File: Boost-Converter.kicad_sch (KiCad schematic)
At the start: 6 parts

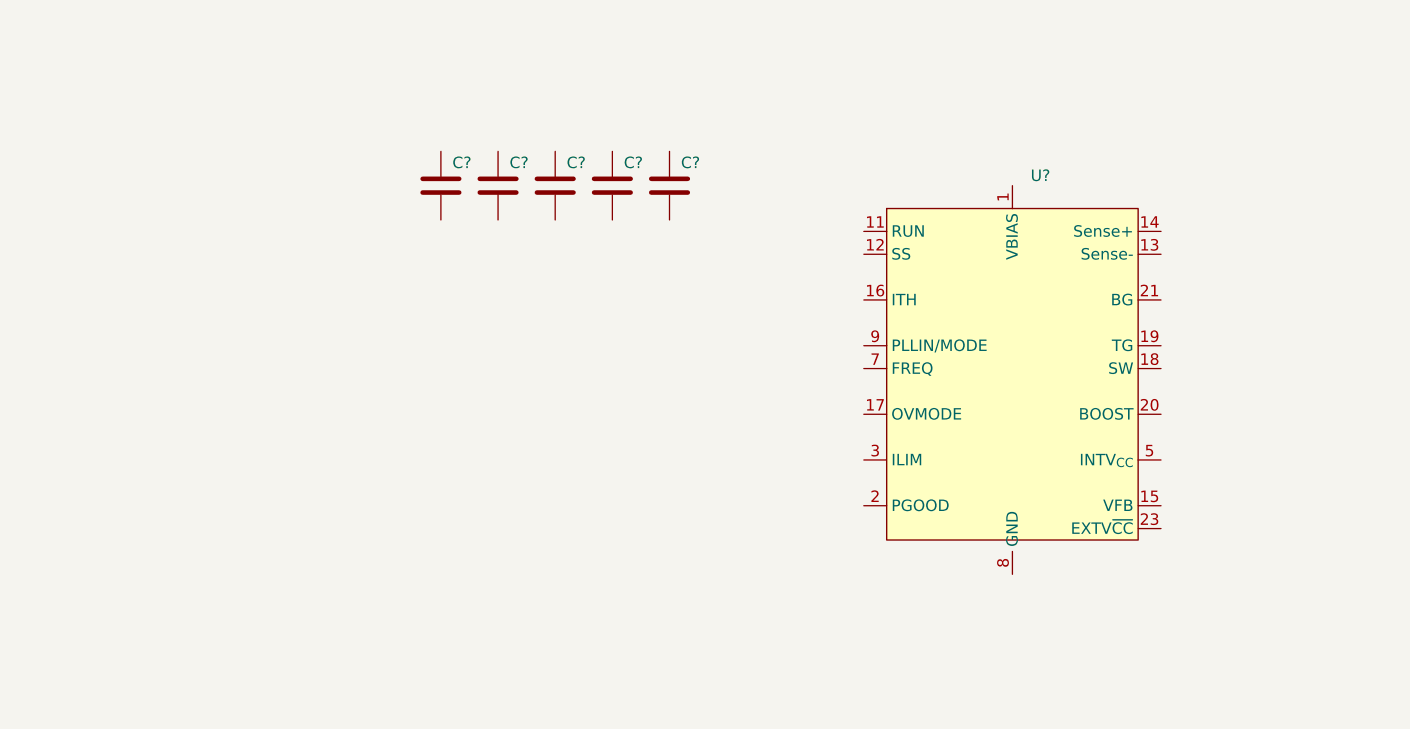
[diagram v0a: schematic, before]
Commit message: WIP boost converter
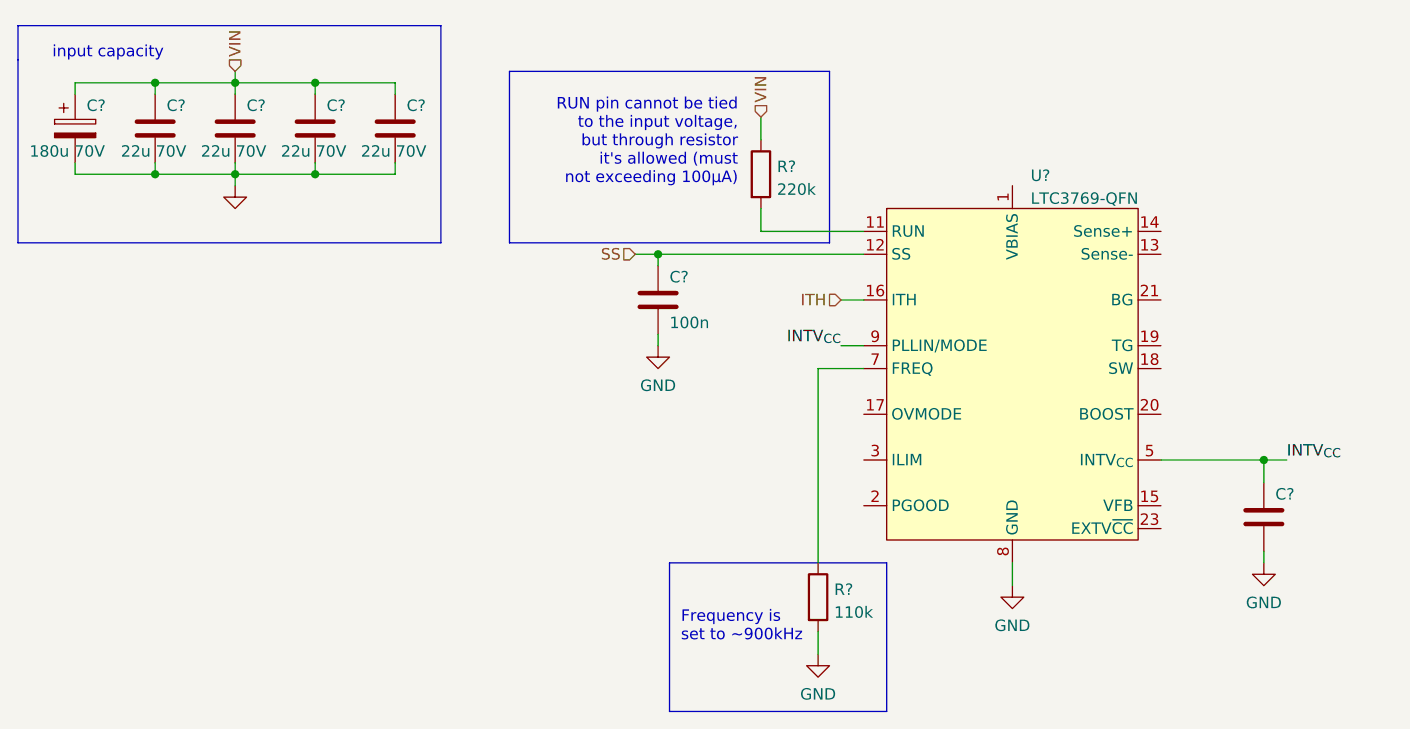
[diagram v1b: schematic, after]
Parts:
- added C?: (no value), symbol Device:C
- added C?: 100n, symbol Device:C
- added R?: 110k, symbol Device:R
- added R?: 220k, symbol Device:R
- C? (x4): value ~ -> 22u 70V
- C?: value (none) -> 180u 70V; symbol Device:C -> Device:C_Polarized
- U?: value (none) -> LTC3769-QFN; footprint (none) -> Package_DFN_QFN:WQFN-24-1EP_4x4mm_P0.5mm_EP2.45x2.45mm_ThermalVias
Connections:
- net VIN: now reaches C?.1
- net VIN: now also C?.1, C?.1, C?.1, C?.1, R?.1
- net GND: now reaches C?.2
- net GND: now also C?.2, C?.2, C?.2, C?.2, U?.10 (GND), U?.24 (GND), U?.25 (GND), U?.8 (GND), C?.2, C?.2, R?.2
- net at U?.11 (RUN): now also R?.2
- net SS: now reaches U?.12 (SS)
- net SS: now also C?.1
- net ITH: now reaches U?.16 (ITH)
- net INTV_{CC}: now reaches U?.22 (INTV_{CC}), U?.5 (INTV_{CC})
- net INTV_{CC}: now also U?.9 (PLLIN/MODE), C?.1
- net at U?.7 (FREQ): now also R?.1
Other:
- note added: "Frequency is set to ~900kHz"
- note added: "RUN pin cannot be tied to the input voltage, but through resistor it's allowed (must not exceeding 100µA)"
- note added: "input capacity"
- moved on the sheet: C?, U?
